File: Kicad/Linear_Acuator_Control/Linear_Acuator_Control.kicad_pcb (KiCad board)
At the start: 2 copper layers, 93.5 x 68 mm, 10 parts, among them K1 RT42xAxx, K3 RT42xAxx, Q1 IRLB3813, Q2 IRLB3813, U1 ESP32-S3-WROOM

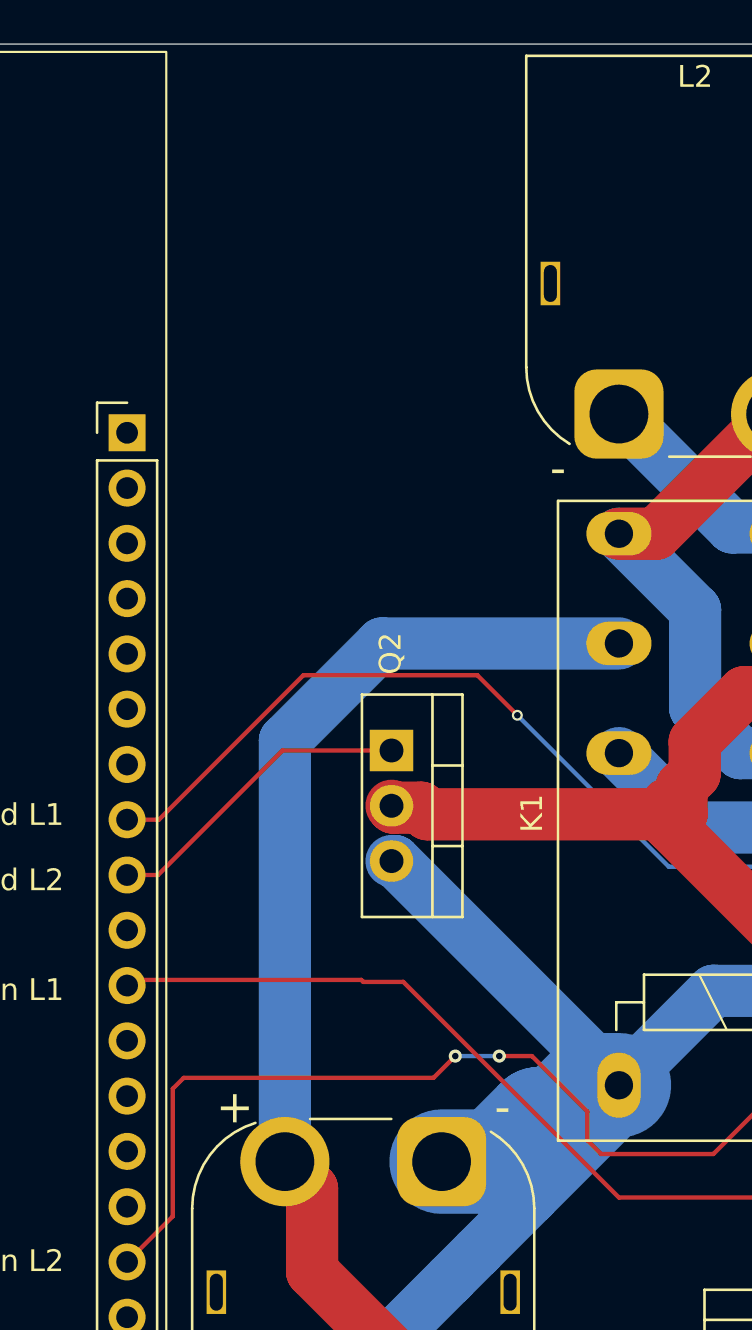
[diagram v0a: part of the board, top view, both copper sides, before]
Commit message: changing things to fix problems
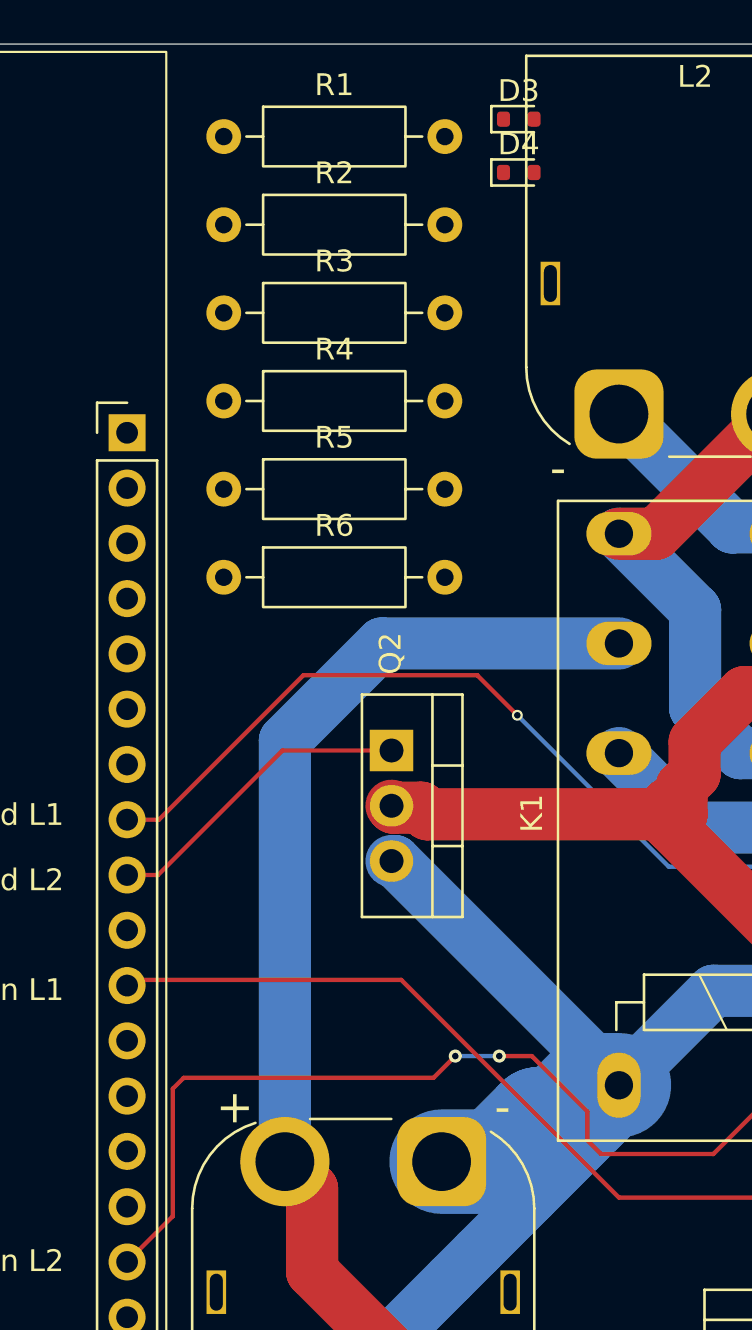
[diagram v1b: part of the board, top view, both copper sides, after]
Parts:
- added D3: 1N4148WT, Diode_SMD:D_SOD-523, F.Cu at (109.9, 40.5)
- added D4: 1N4148WT, Diode_SMD:D_SOD-523, F.Cu at (109.9, 42.9)
- added R1: 1k, Resistor_THT:R_Axial_DIN0207_L6.3mm_D2.5mm_P10.16mm_Horizontal, F.Cu at (96.3, 41.2)
- added R2: 10k, Resistor_THT:R_Axial_DIN0207_L6.3mm_D2.5mm_P10.16mm_Horizontal, F.Cu at (96.3, 45.3)
- added R3: 1k, Resistor_THT:R_Axial_DIN0207_L6.3mm_D2.5mm_P10.16mm_Horizontal, F.Cu at (96.3, 49.4)
- added R4: 10k, Resistor_THT:R_Axial_DIN0207_L6.3mm_D2.5mm_P10.16mm_Horizontal, F.Cu at (96.3, 53.4)
- added R5: 220, Resistor_THT:R_Axial_DIN0207_L6.3mm_D2.5mm_P10.16mm_Horizontal, F.Cu at (96.3, 57.5)
- added R6: 220, Resistor_THT:R_Axial_DIN0207_L6.3mm_D2.5mm_P10.16mm_Horizontal, F.Cu at (96.3, 61.5)
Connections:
- K1 pad A1: Dir L2 -> +24V
- K1 pad A2: GND -> Net-(D4-A)
- K3 pad A1: Dir L1 -> +24V
- K3 pad A2: GND -> Net-(D3-A)
- Q1 pad 1: Speed L1 -> Net-(Q1-G)
- Q2 pad 1: Speed L2 -> Net-(Q2-G)
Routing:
- net unconnected-(U1-GPIO42/MTMS-Pad39): track 0.00 -> 47.5 mm, vias 0 -> 1
- net Speed L1: track 47.5 -> 0.00 mm, vias 1 -> 0
- net +24V: track 129.3 -> 170.7 mm, vias 0 -> 2
- net Dir L2: track 41.4 -> 0.00 mm, vias 2 -> 0
